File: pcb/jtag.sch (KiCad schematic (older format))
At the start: 2 parts, among them J1 CONN_01X10, J2 CONN_01X02

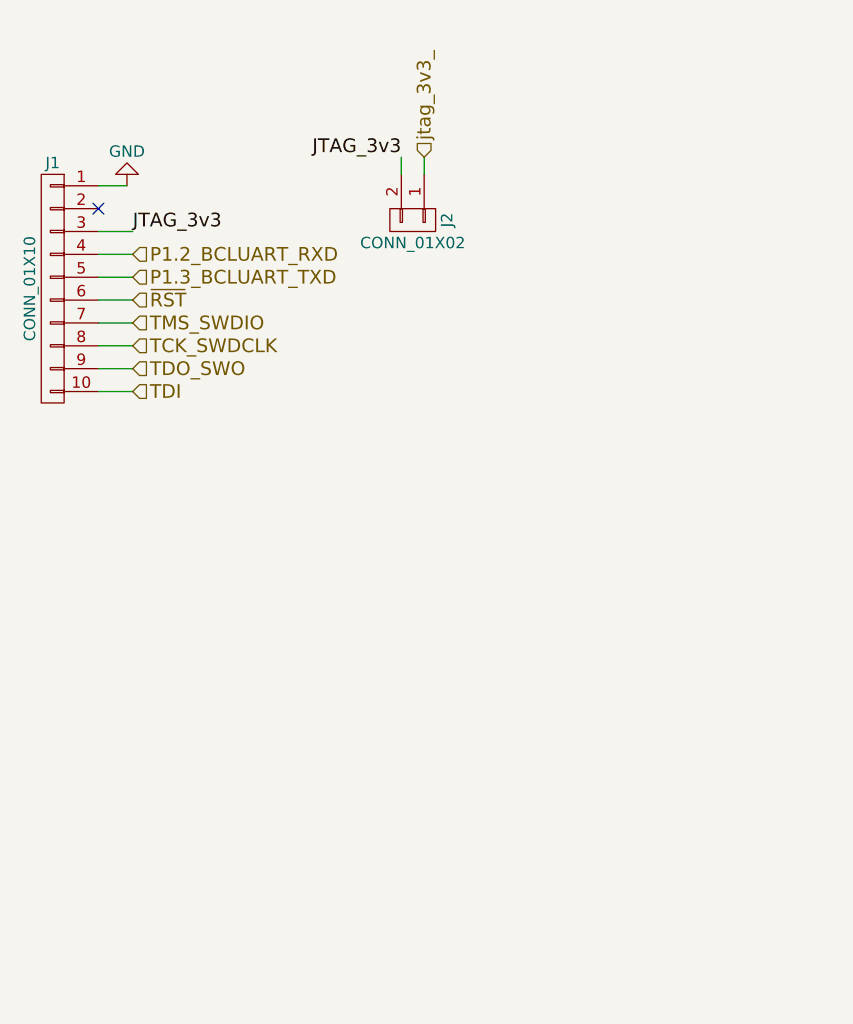
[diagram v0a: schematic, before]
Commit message: Clean up Kicad and TCC
Some changes in the
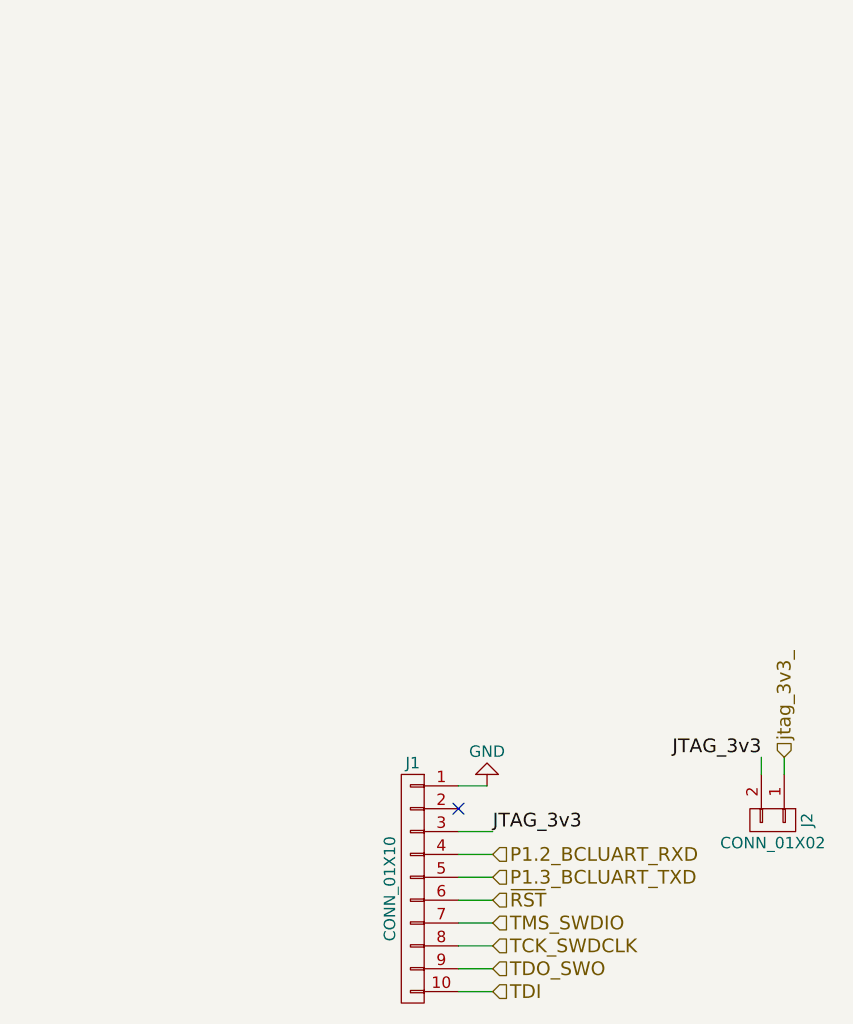
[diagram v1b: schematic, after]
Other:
- moved on the sheet: J1, J2
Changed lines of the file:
@@
 $Descr A4 11693 8268
 encoding utf-8
-Sheet 10 10
-Title ""
+Sheet 9 10
+Title "JTAG Connector Schematic"
 Date ""
-Rev ""
-Comp ""
+Rev "1"
+Comp "Universidade de Brasília - Campus Gama"
 Comment1 ""
 Comment2 ""
@@
 L power:GND #PWR018
 U 1 1 5CD8A9AD
-P 3825 1175
-F 0 "#PWR018" H 3825 925 50  0001 C CNN
-F 1 "GND" H 3825 1025 50  0000 C CNN
-F 2 "" H 3825 1175 50  0001 C CNN
-F 3 "" H 3825 1175 50  0001 C CNN
-	1    3825 1175
+P 5400 3800
+F 0 "#PWR018" H 5400 3550 50  0001 C CNN
+F 1 "GND" H 5400 3650 50  0000 C CNN
+F 2 "" H 5400 3800 50  0001 C CNN
+F 3 "" H 5400 3800 50  0001 C CNN
+	1    5400 3800
 	-1   0    0    1
 $EndComp
@@
 L conn:CONN_01X10 J1
 U 1 1 5CD8ACB1
-P 3500 1625
-F 0 "J1" H 3500 2175 50  0000 C CNN
-F 1 "CONN_01X10" V 3600 1625 50  0000 C CNN
-F 2 "Pin_Headers:Pin_Header_Straight_1x10_Pitch2.54mm" H 3500 1625 50  0001 C CNN
-F 3 "https://www.digikey.com/product-detail/en/amphenol-icc-fci/67997-410HLF/609-3243-ND/1878475" H 3500 1625 50  0001 C CNN
-	1    3500 1625
+P 5075 4250
+F 0 "J1" H 5075 4800 50  0000 C CNN
+F 1 "CONN_01X10" V 5175 4250 50  0000 C CNN
+F 2 "Pin_Headers:Pin_Header_Straight_1x10_Pitch2.54mm" H 5075 4250 50  0001 C CNN
+F 3 "https://www.digikey.com/product-detail/en/amphenol-icc-fci/67997-410HLF/609-3243-ND/1878475" H 5075 4250 50  0001 C CNN
+	1    5075 4250
 	-1   0    0    -1
 $EndComp
 Wire Wire Line
-	3825 1175 3700 1175
+	5400 3800 5275 3800
 $Comp
 L conn:CONN_01X02 J2
 U 1 1 5CD8AD81
-P 5075 1325
-F 0 "J2" H 5075 1475 50  0000 C CNN
-F 1 "CONN_01X02" V 5175 1325 50  0000 C CNN
-F 2 "Pin_Headers:Pin_Header_Straight_1x02_Pitch2.54mm" H 5075 1325 50  0001 C CNN
-F 3 "https://www.digikey.com/product-detail/en/amphenol-icc-fci/67997-410HLF/609-3243-ND/1878475" H 5075 1325 50  0001 C CNN
-	1    5075 1325
+P 6650 3950
+F 0 "J2" H 6650 4100 50  0000 C CNN
+F 1 "CONN_01X02" V 6750 3950 50  0000 C CNN
+F 2 "Pin_Headers:Pin_Header_Straight_1x02_Pitch2.54mm" H 6650 3950 50  0001 C CNN
+F 3 "https://www.digikey.com/product-detail/en/amphenol-icc-fci/67997-410HLF/609-3243-ND/1878475" H 6650 3950 50  0001 C CNN
+	1    6650 3950
 	0    1    1    0
 $EndComp
-Text Label 3850 1375 0    60   ~ 0
+Text Label 5425 4000 0    60   ~ 0
 JTAG_3v3
 Wire Wire Line
-	3850 1375 3700 1375
-Text HLabel 3850 1475 2    60   Input ~ 0
+	5425 4000 5275 4000
+Text HLabel 5425 4100 2    60   Input ~ 0
 P1.2_BCLUART_RXD
 Wire Wire Line
-	3850 1475 3700 1475
-Text HLabel 3850 1575 2    60   Input ~ 0
+	5425 4100 5275 4100
+Text HLabel 5425 4200 2    60   Input ~ 0
 P1.3_BCLUART_TXD
 Wire Wire Line
-	3850 1575 3700 1575
-Text Label 5025 1050 2    60   ~ 0
+	5425 4200 5275 4200
+Text Label 6600 3675 2    60   ~ 0
 JTAG_3v3
 Wire Wire Line
-	5025 1050 5025 1125
-Text HLabel 3850 1675 2    60   Input ~ 0
+	6600 3675 6600 3750
+Text HLabel 5425 4300 2    60   Input ~ 0
 ~RST
 Wire Wire Line
-	3850 1675 3700 1675
-Text HLabel 3850 1775 2    60   Input ~ 0
+	5425 4300 5275 4300
+Text HLabel 5425 4400 2    60   Input ~ 0
 TMS_SWDIO
-Text HLabel 3850 1875 2    60   Input ~ 0
+Text HLabel 5425 4500 2    60   Input ~ 0
 TCK_SWDCLK
-Text HLabel 3850 1975 2    60   Input ~ 0
+Text HLabel 5425 4600 2    60   Input ~ 0
 TDO_SWO
-Text HLabel 3850 2075 2    60   Input ~ 0
+Text HLabel 5425 4700 2    60   Input ~ 0
 TDI
 Wire Wire Line
-	3850 2075 3700 2075
+	5425 4700 5275 4700
 Wire Wire Line
-	3700 1975 3850 1975
+	5275 4600 5425 4600
 Wire Wire Line
-	3700 1875 3850 1875
+	5275 4500 5425 4500
 Wire Wire Line
-	3700 1775 3850 1775
-Text HLabel 5125 1050 1    60   Input ~ 0
+	5275 4400 5425 4400
+Text HLabel 6700 3675 1    60   Input ~ 0
 jtag_3v3_
 Wire Wire Line
-	5125 1050 5125 1125
-NoConn ~ 3700 1275
+	6700 3675 6700 3750
+NoConn ~ 5275 3900
 $EndSCHEMATC
